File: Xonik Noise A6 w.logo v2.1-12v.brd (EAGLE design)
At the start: 29.8 x 26 mm, 39 parts, among them IC1 TL074D, T1 NOISE-2N3904

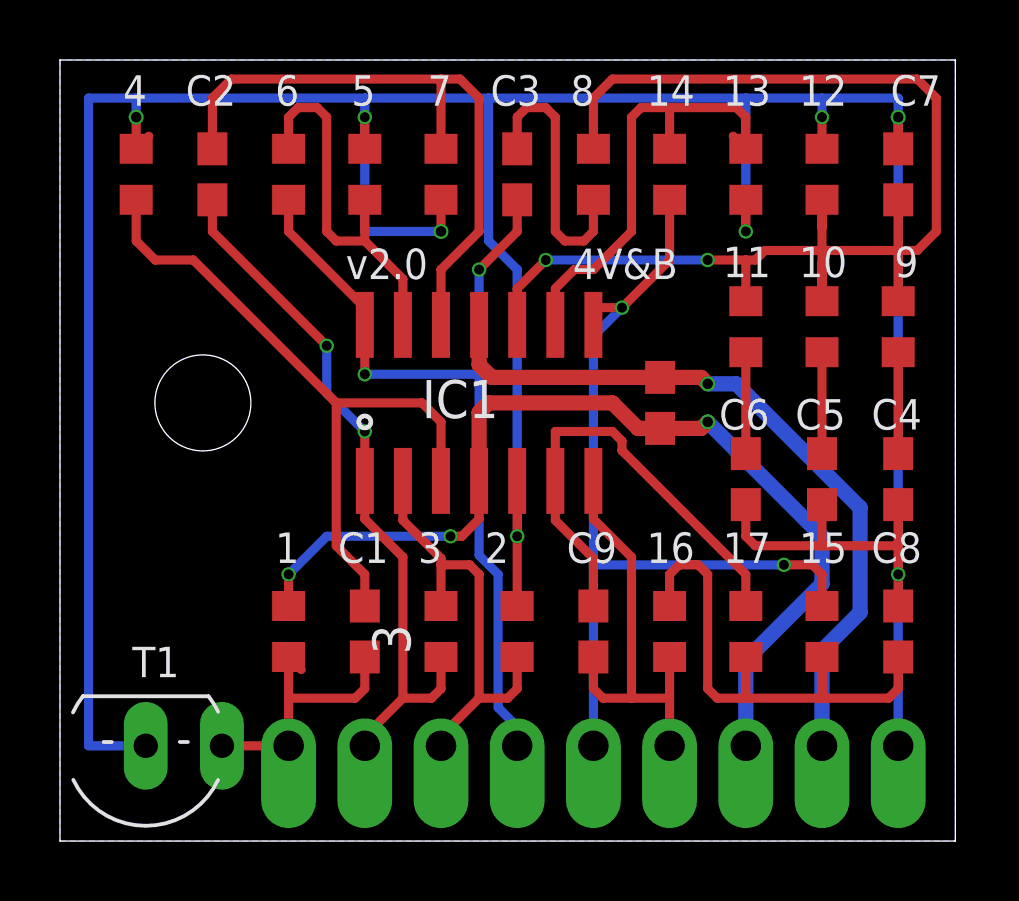
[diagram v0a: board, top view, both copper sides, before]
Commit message: Version 2.1 12V completed I think
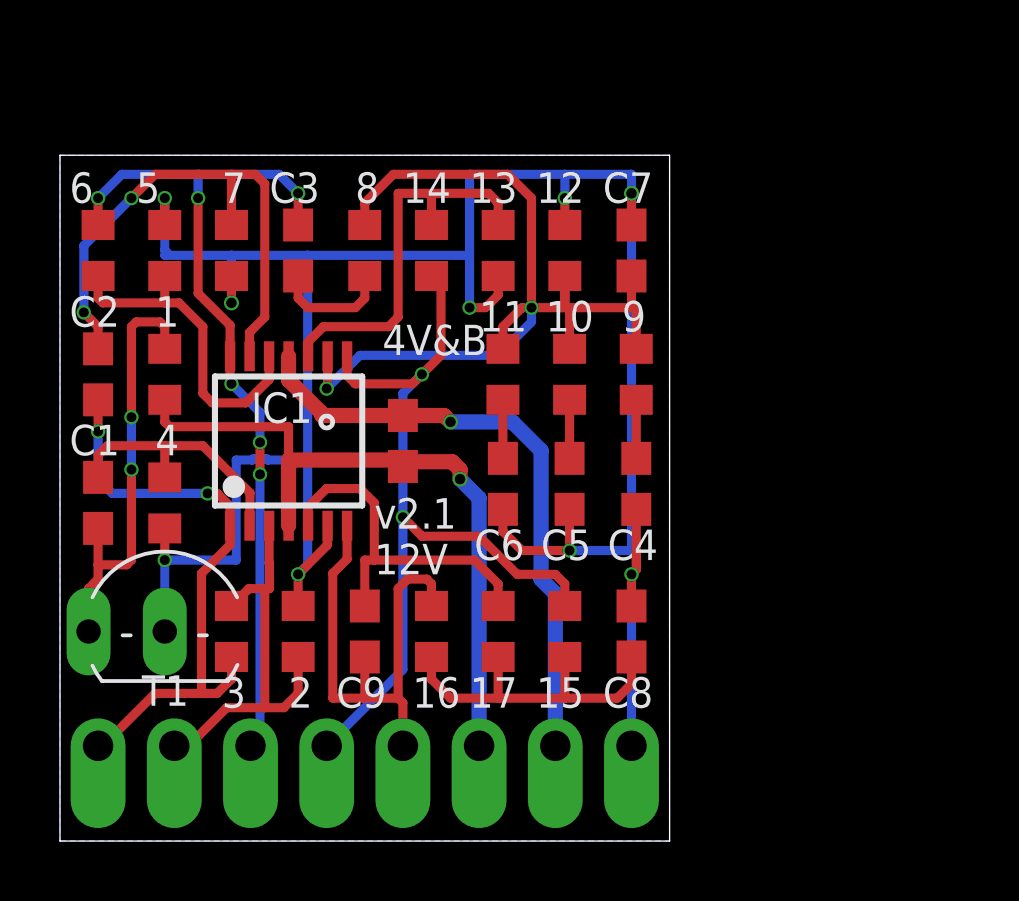
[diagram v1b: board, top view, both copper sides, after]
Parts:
- removed NOISE_IN: (no value), joakim:SIP-PIN01-1J
- IC1: value TL074D -> TL074JT; device linear:SO14 -> joakim:TSSOP14J
- moved 4 11.0 mm to (3.49, 11.3), turned to 270 degrees
- moved C1 9.87 mm to (1.27, 11.3)
- moved 1 9.51 mm to (3.49, 15.6), turned to 270 degrees
- moved C7 9.25 mm to (19.1, 19.7)
- moved 12 8.94 mm to (16.8, 19.7)
- moved C8 8.89 mm to (19.1, 6.99)
- moved GND 8.89 mm to (19.1, 3.17)
- moved LEVEL2 8.89 mm to (1.27, 3.17)
- moved PINK_OUT 8.89 mm to (8.89, 3.17)
- moved RED_OUT 8.89 mm to (11.4, 3.17)
- moved WHITE_OUT 8.89 mm to (6.35, 3.17)
- moved +15V 8.89 mm to (14.0, 3.17)
- moved LEVEL1 8.89 mm to (3.81, 3.17)
- moved -15V 8.89 mm to (16.5, 3.17)
- moved 9 8.87 mm to (19.2, 15.6)
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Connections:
- net GND: now also IC1.6; no longer IC1.5
- net N$1: now also IC1.3; no longer IC1.2
- net N$10: now also IC1.13; no longer IC1.12
- net N$12: now also IC1.9; no longer IC1.10
- net N$17: now also IC1.5; no longer IC1.6
- net N$2: now also IC1.12; no longer IC1.13
- net N$3: now also IC1.10; no longer IC1.9
- net N$7: no longer NOISE_IN.1
- net N$8: now also IC1.2; no longer IC1.3
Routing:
- net GND: track 123.7 -> 84.5 mm, vias 8 -> 9
- net N$8: track 23.4 -> 8.73 mm
- net N$12: track 44.4 -> 31.4 mm
- net +12V: track 33.3 -> 23.8 mm, vias 3 -> 1
- net N$16: track 18.6 -> 11.5 mm
- net N$13: track 9.93 -> 3.96 mm
- net N$7: track 9.92 -> 14.5 mm, vias 0 -> 2
- net -12V: track 24.5 -> 20.3 mm
- net N$17: track 15.9 -> 12.2 mm
- net N$9: track 23.8 -> 20.2 mm
- net N$10: track 21.5 -> 18.4 mm, vias 0 -> 2
- net N$3: track 16.2 -> 13.2 mm
- net N$18: track 14.7 -> 16.8 mm
- net N$14: track 29.7 -> 27.8 mm
- net N$2: track 13.0 -> 11.2 mm
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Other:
- board size 29.8 x 26 mm -> 20.3 x 22.9 mm
- board text added: "+12V"
- board text added: "-12V"
- board text added: "Trim"
- board text added: "v2.1 12V"
- board text removed: "+15V"
- board text removed: "-15V"
- board text removed: "1"
- board text removed: "10"
- board text removed: "11"
- board text removed: "12"
- board text removed: "13"
- board text removed: "14"
- board text removed: "15"
- board text removed: "16"
- board text removed: "17"
- board text removed: "2"
- board text removed: "3"
- board text removed: "4"
- board text removed: "5"
- board text removed: "50k Trim"
- board text removed: "6"
- board text removed: "7"
- board text removed: "8"
- board text removed: "9"
- board text removed: "C1"
- board text removed: "C2"
- board text removed: "C3"
- board text removed: "C4"
- board text removed: "C5"
- board text removed: "C6"
- board text removed: "C7"
- board text removed: "C8"
- board text removed: "C9"
- board text removed: "In"
- board text removed: "v2.0"
